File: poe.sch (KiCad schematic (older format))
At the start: 15 parts

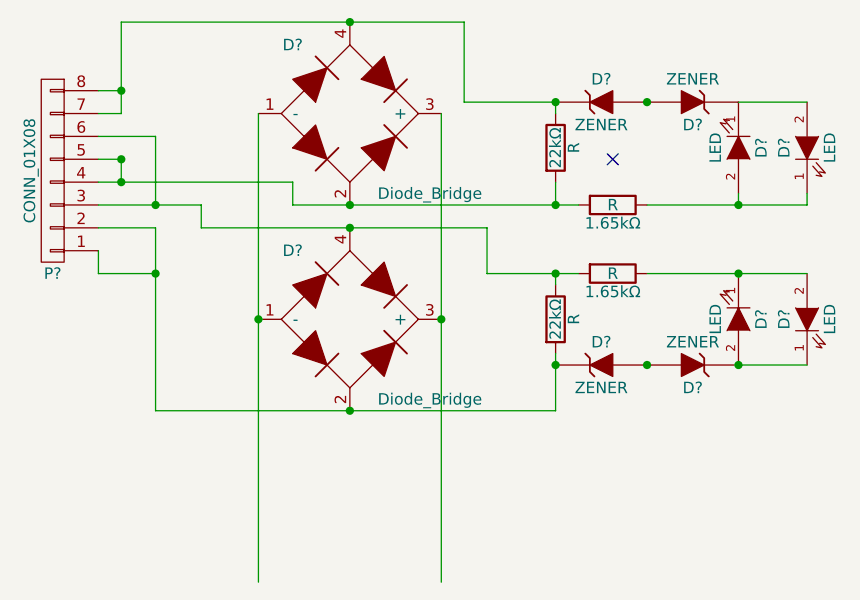
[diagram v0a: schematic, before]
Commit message: am Routing rumgespielt
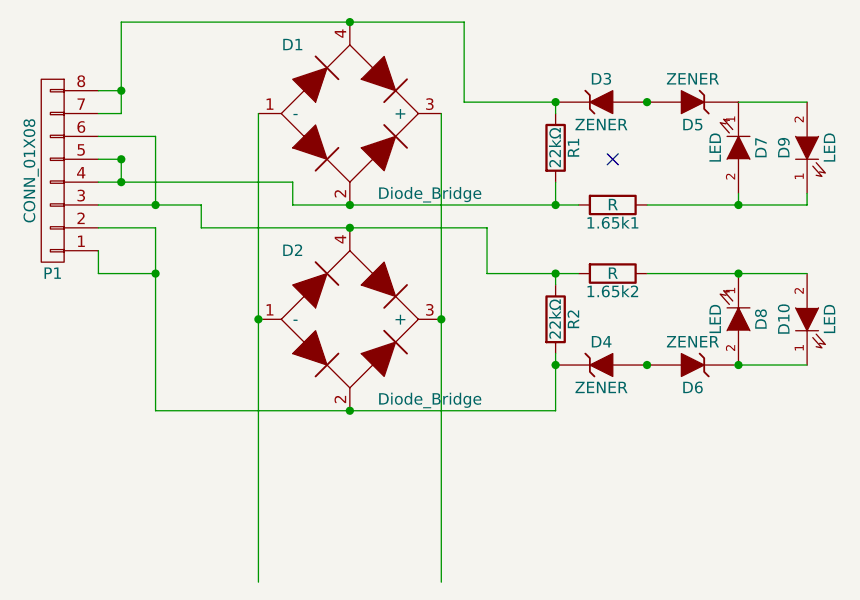
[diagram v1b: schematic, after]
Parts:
- 1.65k1, 1.65k2: renamed from 1.65kΩ; footprint (none) -> Resistors_ThroughHole:Resistor_Horizontal_RM20mm
- D1, D2: renamed from D?; footprint (none) -> Diodes_ThroughHole:Diode_DO-35_SOD27_Horizontal_RM10
- D10, D7, D8, D9: renamed from D?; footprint (none) -> LEDs:LED-3MM
- D3, D4, D5, D6: renamed from D?; footprint (none) -> Discret:D3
- P1: renamed from P?; footprint (none) -> Pin_Headers:Pin_Header_Angled_1x08
- R1, R2: renamed from R; footprint (none) -> Resistors_ThroughHole:Resistor_Horizontal_RM7mm
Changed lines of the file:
@@
 $EndDescr
 $Comp
-L CONN_01X08 P?
+L CONN_01X08 P1
 U 1 1 589CD597
 P 3300 3150
-F 0 "P?" H 3300 3600 50  0000 C CNN
+F 0 "P1" H 3300 3600 50  0000 C CNN
 F 1 "CONN_01X08" V 3400 3150 50  0000 C CNN
-F 2 "" H 3300 3150 50  0000 C CNN
+F 2 "Pin_Headers:Pin_Header_Angled_1x08" H 3300 3150 50  0001 C CNN
 F 3 "" H 3300 3150 50  0000 C CNN
 	1    3300 3150
@@
 $EndComp
 $Comp
-L R R
+L R R1
 U 1 1 589CD7AC
 P 5500 3050
-F 0 "R" V 5580 3050 50  0000 C CNN
+F 0 "R1" V 5580 3050 50  0000 C CNN
 F 1 "22kΩ" V 5500 3050 50  0000 C CNN
-F 2 "" V 5430 3050 50  0000 C CNN
+F 2 "Resistors_ThroughHole:Resistor_Horizontal_RM7mm" V 5430 3050 50  0001 C CNN
 F 3 "" H 5500 3050 50  0000 C CNN
 	1    5500 3050
@@
 $EndComp
 $Comp
-L R R
+L R R2
 U 1 1 589CD7FF
 P 5500 3800
-F 0 "R" V 5580 3800 50  0000 C CNN
+F 0 "R2" V 5580 3800 50  0000 C CNN
 F 1 "22kΩ" V 5500 3800 50  0000 C CNN
-F 2 "" V 5430 3800 50  0000 C CNN
+F 2 "Resistors_ThroughHole:Resistor_Horizontal_RM7mm" V 5430 3800 50  0001 C CNN
 F 3 "" H 5500 3800 50  0000 C CNN
 	1    5500 3800
@@
 $EndComp
 $Comp
-L ZENER D?
+L ZENER D4
 U 1 1 589CDF37
 P 5700 4000
-F 0 "D?" H 5700 4100 50  0000 C CNN
+F 0 "D4" H 5700 4100 50  0000 C CNN
 F 1 "ZENER" H 5700 3900 50  0000 C CNN
-F 2 "" H 5700 4000 50  0000 C CNN
+F 2 "Discret:D3" H 5700 4000 50  0001 C CNN
 F 3 "" H 5700 4000 50  0000 C CNN
 	1    5700 4000
@@
 $EndComp
 $Comp
-L ZENER D?
+L ZENER D6
 U 1 1 589CE16F
 P 6100 4000
-F 0 "D?" H 6100 4100 50  0000 C CNN
+F 0 "D6" H 6100 4100 50  0000 C CNN
 F 1 "ZENER" H 6100 3900 50  0000 C CNN
-F 2 "" H 6100 4000 50  0000 C CNN
+F 2 "Discret:D3" H 6100 4000 50  0001 C CNN
 F 3 "" H 6100 4000 50  0000 C CNN
 	1    6100 4000
@@
 $EndComp
 $Comp
-L ZENER D?
+L ZENER D3
 U 1 1 589CE1DE
 P 5700 2850
-F 0 "D?" H 5700 2950 50  0000 C CNN
+F 0 "D3" H 5700 2950 50  0000 C CNN
 F 1 "ZENER" H 5700 2750 50  0000 C CNN
-F 2 "" H 5700 2850 50  0000 C CNN
+F 2 "Discret:D3" H 5700 2850 50  0001 C CNN
 F 3 "" H 5700 2850 50  0000 C CNN
 	1    5700 2850
@@
 $EndComp
 $Comp
-L ZENER D?
+L ZENER D5
 U 1 1 589CE247
 P 6100 2850
-F 0 "D?" H 6100 2950 50  0000 C CNN
+F 0 "D5" H 6100 2950 50  0000 C CNN
 F 1 "ZENER" H 6100 2750 50  0000 C CNN
-F 2 "" H 6100 2850 50  0000 C CNN
+F 2 "Discret:D3" H 6100 2850 50  0001 C CNN
 F 3 "" H 6100 2850 50  0000 C CNN
 	1    6100 2850
@@
 $EndComp
 $Comp
-L R 1.65kΩ
+L R 1.65k1
 U 1 1 589CE2D4
 P 5750 3300
-F 0 "1.65kΩ" V 5830 3300 50  0000 C CNN
+F 0 "1.65k1" V 5830 3300 50  0000 C CNN
 F 1 "R" V 5750 3300 50  0000 C CNN
-F 2 "" V 5680 3300 50  0000 C CNN
+F 2 "Resistors_ThroughHole:Resistor_Horizontal_RM20mm" V 5680 3300 50  0001 C CNN
 F 3 "" H 5750 3300 50  0000 C CNN
 	1    5750 3300
@@
 $EndComp
 $Comp
-L R 1.65kΩ
+L R 1.65k2
 U 1 1 589CE307
 P 5750 3600
-F 0 "1.65kΩ" V 5830 3600 50  0000 C CNN
+F 0 "1.65k2" V 5830 3600 50  0000 C CNN
 F 1 "R" V 5750 3600 50  0000 C CNN
-F 2 "" V 5680 3600 50  0000 C CNN
+F 2 "Resistors_ThroughHole:Resistor_Horizontal_RM20mm" V 5680 3600 50  0001 C CNN
 F 3 "" H 5750 3600 50  0000 C CNN
 	1    5750 3600
@@
 $EndComp
 $Comp
-L LED D?
+L LED D8
 U 1 1 589CE453
 P 6300 3800
-F 0 "D?" H 6300 3900 50  0000 C CNN
+F 0 "D8" H 6300 3900 50  0000 C CNN
 F 1 "LED" H 6300 3700 50  0000 C CNN
-F 2 "" H 6300 3800 50  0000 C CNN
+F 2 "LEDs:LED-3MM" H 6300 3800 50  0001 C CNN
 F 3 "" H 6300 3800 50  0000 C CNN
 	1    6300 3800
@@
 $EndComp
 $Comp
-L LED D?
+L LED D10
 U 1 1 589CE49E
 P 6600 3800
-F 0 "D?" H 6600 3900 50  0000 C CNN
+F 0 "D10" H 6600 3900 50  0000 C CNN
 F 1 "LED" H 6600 3700 50  0000 C CNN
-F 2 "" H 6600 3800 50  0000 C CNN
+F 2 "LEDs:LED-3MM" H 6600 3800 50  0001 C CNN
 F 3 "" H 6600 3800 50  0000 C CNN
 	1    6600 3800
@@
 $EndComp
 $Comp
-L LED D?
+L LED D7
 U 1 1 589CE770
 P 6300 3050
-F 0 "D?" H 6300 3150 50  0000 C CNN
+F 0 "D7" H 6300 3150 50  0000 C CNN
 F 1 "LED" H 6300 2950 50  0000 C CNN
-F 2 "" H 6300 3050 50  0000 C CNN
+F 2 "LEDs:LED-3MM" H 6300 3050 50  0001 C CNN
 F 3 "" H 6300 3050 50  0000 C CNN
 	1    6300 3050
@@
 $EndComp
 $Comp
-L LED D?
+L LED D9
 U 1 1 589CE7ED
 P 6600 3050
-F 0 "D?" H 6600 3150 50  0000 C CNN
+F 0 "D9" H 6600 3150 50  0000 C CNN
 F 1 "LED" H 6600 2950 50  0000 C CNN
-F 2 "" H 6600 3050 50  0000 C CNN
+F 2 "LEDs:LED-3MM" H 6600 3050 50  0001 C CNN
 F 3 "" H 6600 3050 50  0000 C CNN
 	1    6600 3050
@@
 	6600 2850 6300 2850
 $Comp
-L Diode_Bridge D?
+L Diode_Bridge D1
 U 1 1 58A4AC46
 P 4600 2900
-F 0 "D?" H 4350 3200 50  0000 C CNN
+F 0 "D1" H 4350 3200 50  0000 C CNN
 F 1 "Diode_Bridge" H 4950 2550 50  0000 C CNN
-F 2 "" H 4600 2900 50  0000 C CNN
+F 2 "Diodes_ThroughHole:Diode_DO-35_SOD27_Horizontal_RM10" H 4600 2900 50  0001 C CNN
 F 3 "" H 4600 2900 50  0000 C CNN
 	1    4600 2900
@@
 	3600 3100 3600 3200
 $Comp
-L Diode_Bridge D?
+L Diode_Bridge D2
 U 1 1 58A4B96E
 P 4600 3800
-F 0 "D?" H 4350 4100 50  0000 C CNN
+F 0 "D2" H 4350 4100 50  0000 C CNN
 F 1 "Diode_Bridge" H 4950 3450 50  0000 C CNN
-F 2 "" H 4600 3800 50  0000 C CNN
+F 2 "Diodes_ThroughHole:Diode_DO-35_SOD27_Horizontal_RM10" H 4600 3800 50  0001 C CNN
 F 3 "" H 4600 3800 50  0000 C CNN
 	1    4600 3800
